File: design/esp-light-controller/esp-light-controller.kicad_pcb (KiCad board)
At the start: 4 copper layers, 50 x 57.6 mm, 42 parts, among them J1 LED0, J2 LED1, J3 LED2, J4 UART, P1 USB_C_Plug_USB2.0, Q1 2N7002, Q2 2N7002, Q3 2N7002, Q4 2N7002, Q5 2N7002, SW1 RST, SW2 BOOT, U1 CP2104, U2 AMS1117-3.3, U3 ESP32-WROOM-32

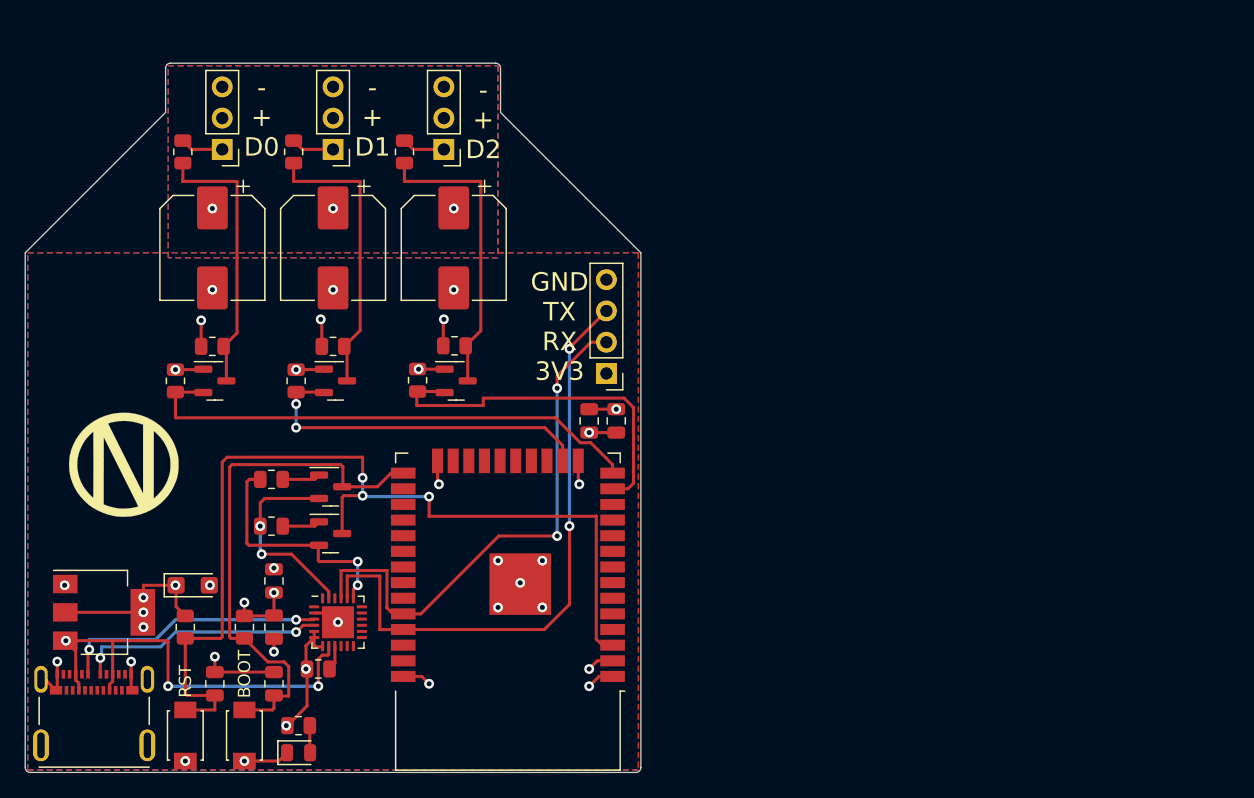
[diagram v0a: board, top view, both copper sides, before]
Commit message: update
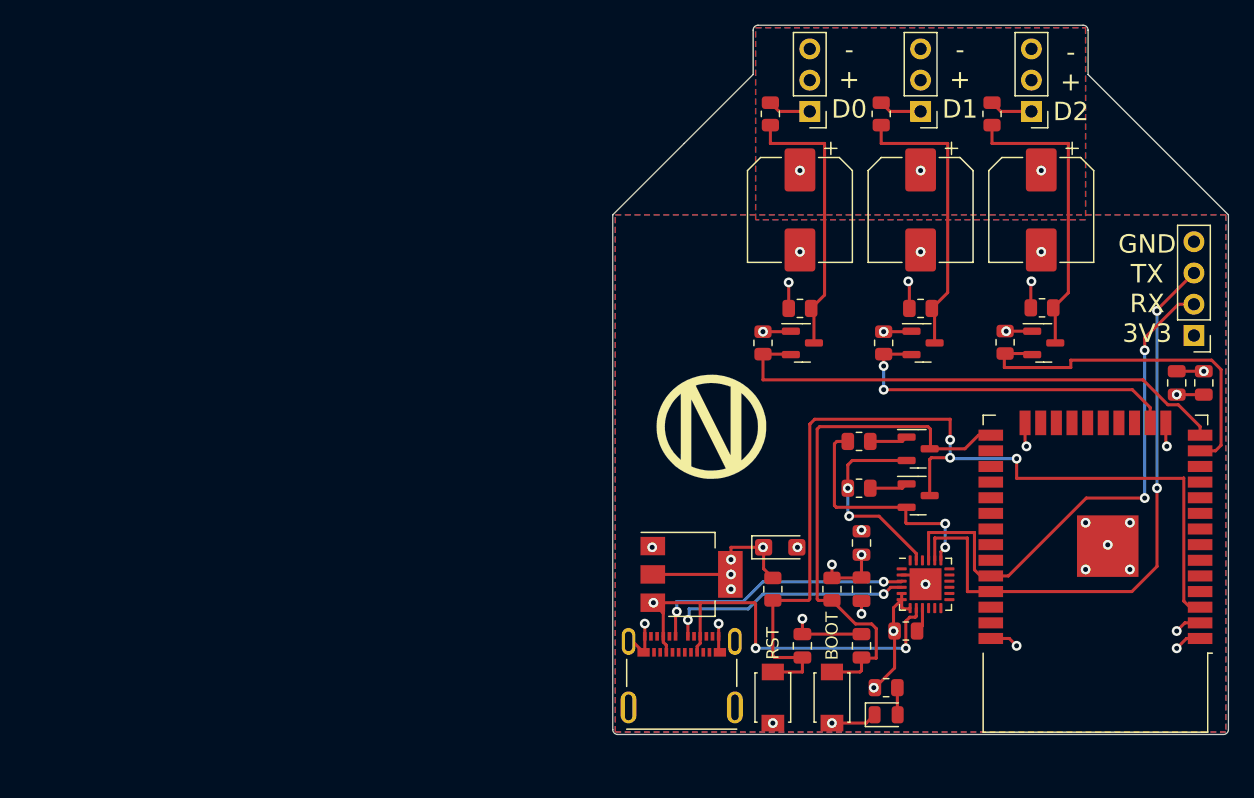
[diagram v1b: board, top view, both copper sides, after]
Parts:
- moved C5 47.8 mm to (160.9, 77.0)
- moved C8 47.8 mm to (149.9, 63.0)
- moved Q4 47.8 mm to (139.9, 86.2)
- moved Q5 47.8 mm to (139.9, 82.4)
- moved R1 47.8 mm to (138.9, 97.2)
- moved R14 47.8 mm to (136.9, 55.2)
- moved R15 47.8 mm to (145.9, 55.2)
- moved R3 47.8 mm to (146.9, 73.7)
- moved R6 47.8 mm to (149.9, 70.9)
- moved R8 47.8 mm to (132.9, 93.8)
- moved SW2 47.8 mm to (132.9, 102.6)
- moved C3 47.8 mm to (163.1, 77.0)
- moved C4 47.8 mm to (128.7, 90.4)
- moved C6 47.8 mm to (130.5, 98.4)
- moved C9 47.8 mm to (140.1, 63.0)
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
